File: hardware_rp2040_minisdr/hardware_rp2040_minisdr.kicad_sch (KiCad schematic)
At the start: 48 parts, among them IC1 PSA4-5043+, IC2 ADE-11X+, IC3 SI5351A-B-GTR, IC4 GALI-84+, IC5 ADCS7476AIMFX_NOPB, J1 Conn_Coaxial_Small, J2 USB_A, SW1 SW_Push, U1 RP2040, U2 W25Q128JVS, U3 AMS1117-3.3, Y1 Crystal_GND24, Y2 Crystal_GND24

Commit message: LEDs
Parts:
- J2: footprint (none) -> user_imported_devices:USBPCB
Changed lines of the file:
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@@
 			)
 		)
-		(property "Footprint" ""
+		(property "Footprint" "user_imported_devices:USBPCB"
 			(at 44.45 52.07 0)
 			(effects

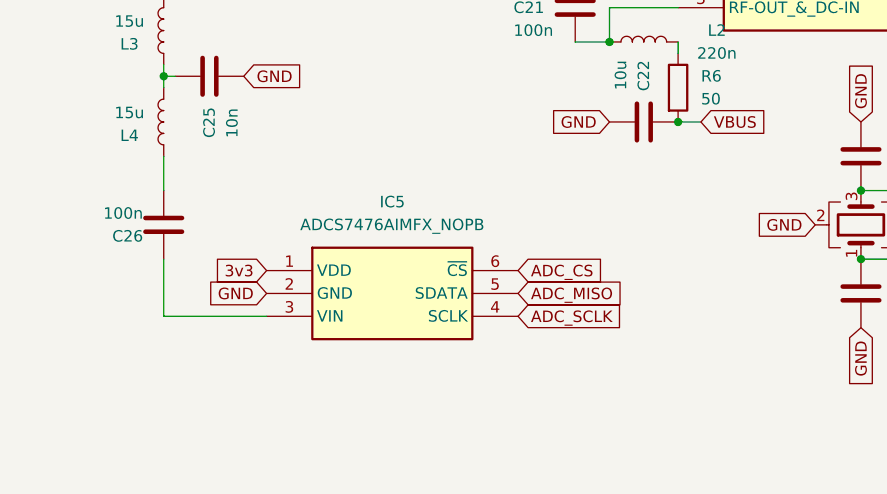
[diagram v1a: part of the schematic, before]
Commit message: board
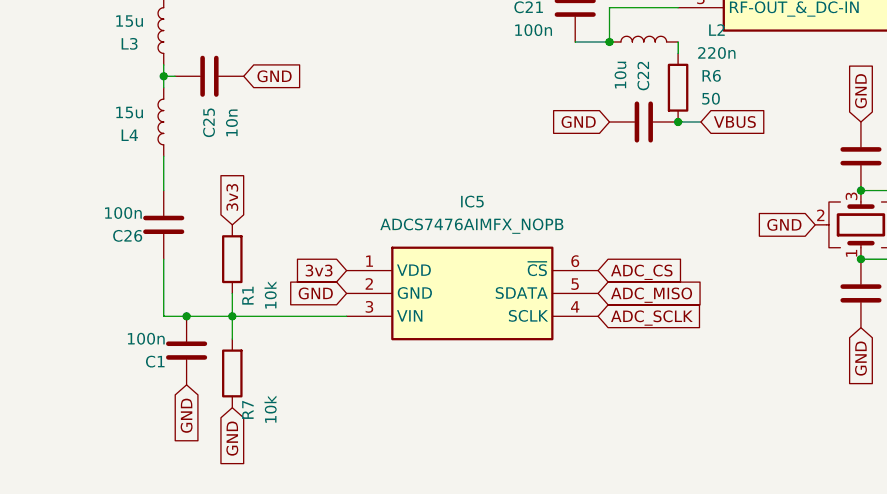
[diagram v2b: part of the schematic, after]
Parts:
- added C1: 100n, Capacitor_SMD:C_0402_1005Metric, symbol Device:C
- added R1, R7: 10k, Resistor_SMD:R_0402_1005Metric, symbol Device:R
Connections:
- net 3v3: now also R1.2
- net GND: now also C1.1, R7.1
- net at C26.1, IC5.3 (VIN): now also C1.2, R1.1, R7.2
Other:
- moved on the sheet: IC5
